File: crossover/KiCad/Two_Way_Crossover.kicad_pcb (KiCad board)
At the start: 2 copper layers, 116.8 x 152.4 mm, 21 parts, among them J1 Conn_01x01_Female, J2 Conn_01x01_Female, J3 Woofer, J4 Tweeter

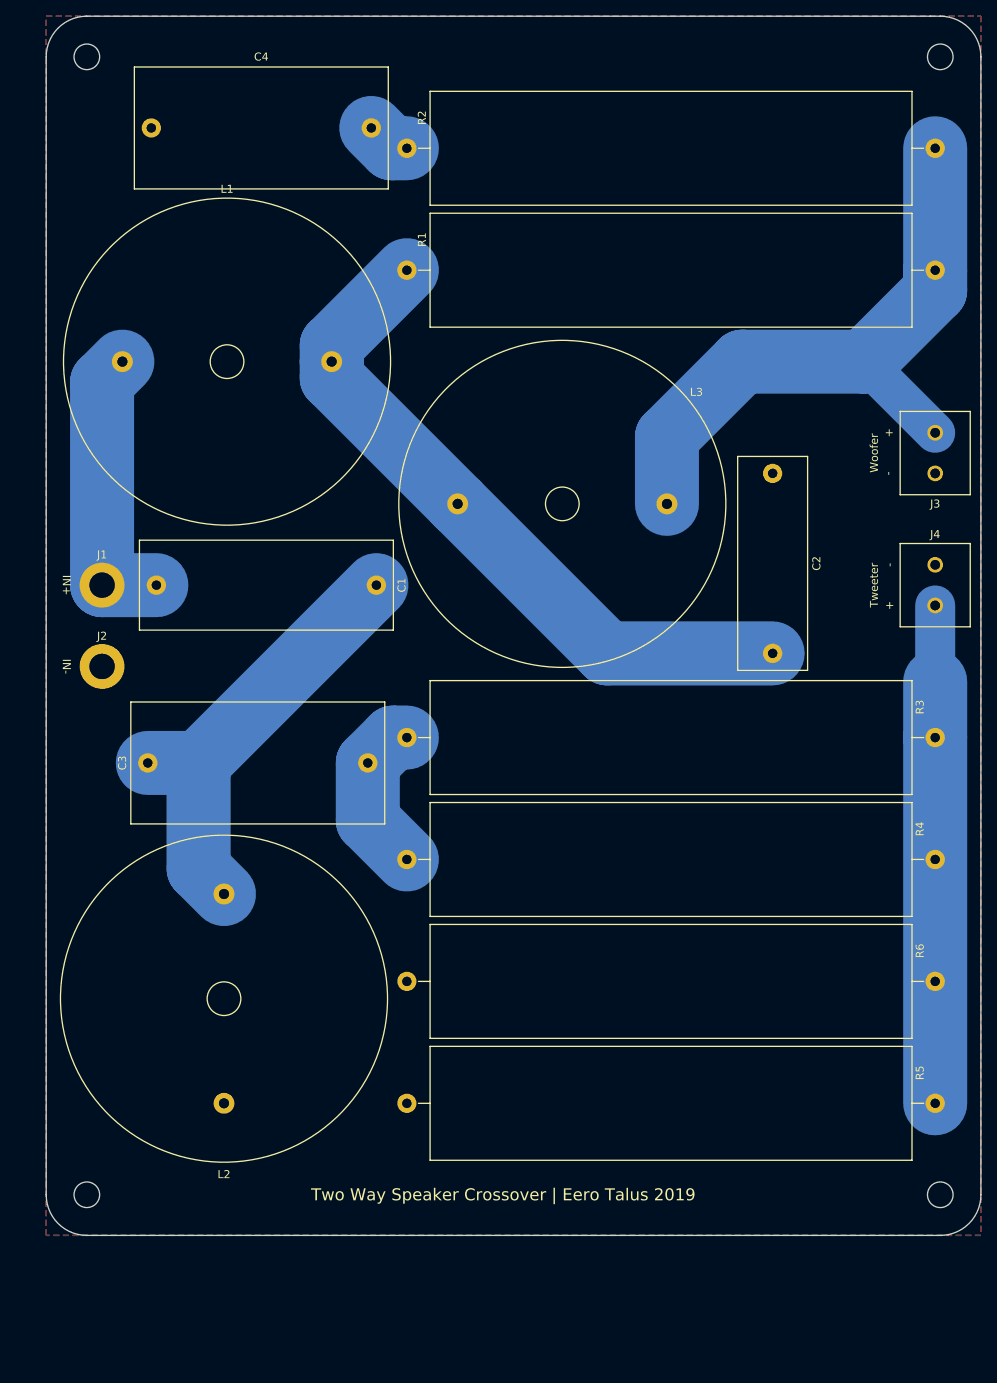
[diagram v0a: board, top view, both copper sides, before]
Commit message: Redesign PCB
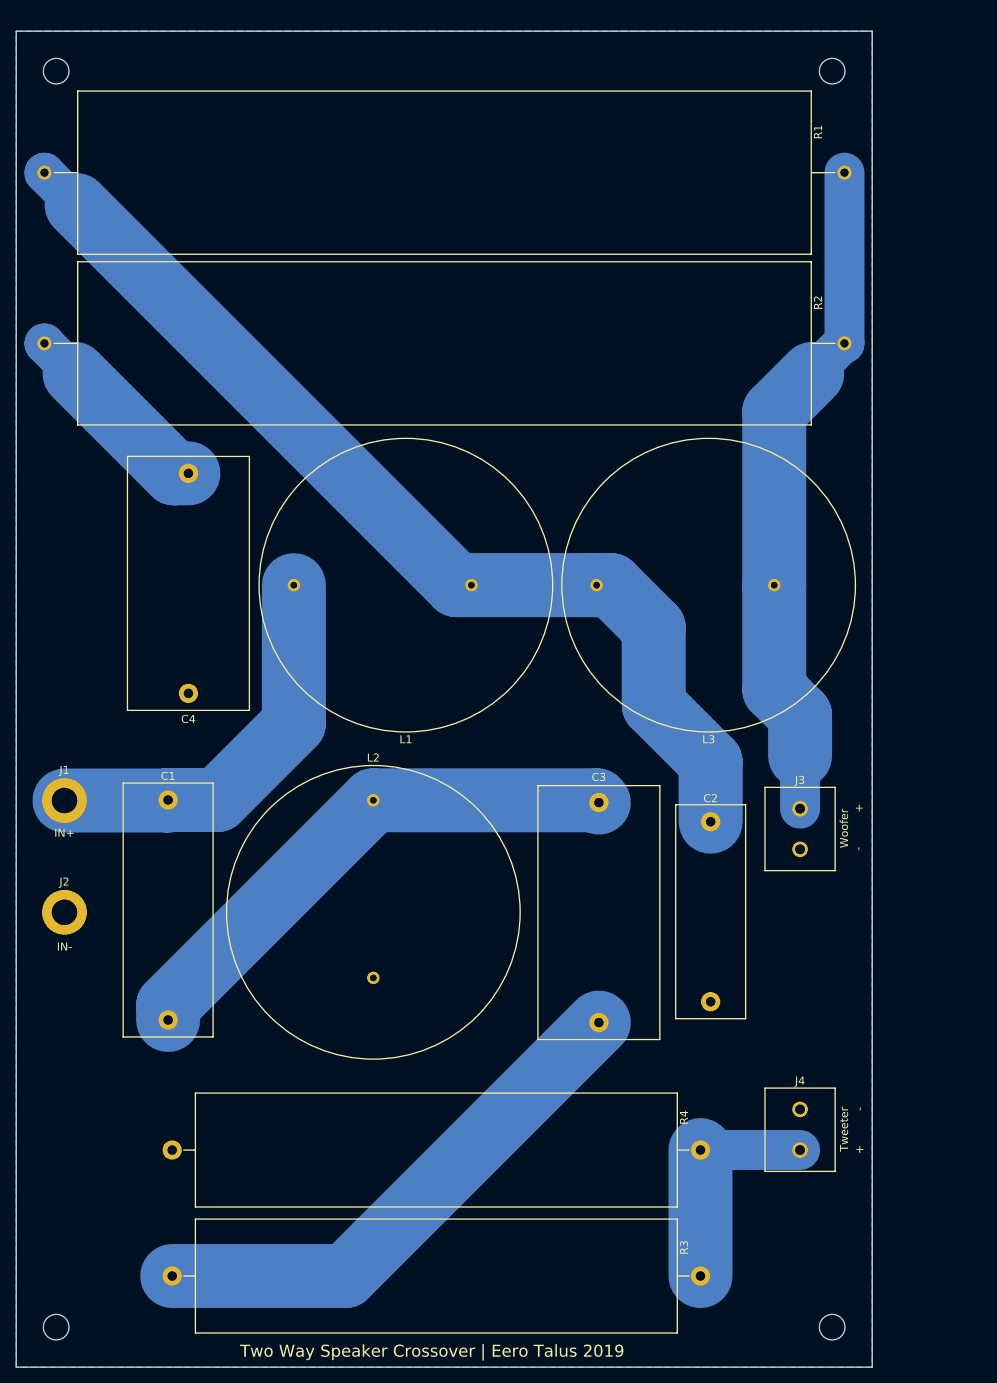
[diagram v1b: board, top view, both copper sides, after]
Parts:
- removed R5, R6: 8R2, Resistor_THT:R_Axial_Power_L60.0mm_W14.0mm_P66.04mm
- L1, L2, L3: footprint Inductor_THT:L_Radial_D40.6mm_P26.16mm_Vishay_IHB-5 -> etal_Inductors:Radial_D36.5mm_H12.0mm_P23.0mm
- R1, R2: footprint Resistor_THT:R_Axial_Power_L60.0mm_W14.0mm_P66.04mm -> etal_Power_Resistor:Resistor_Power_Axial_L91.5_W20.2_H20.2
- R3, R4: value 8R2 -> 4R7
- moved H1 110.5 mm to (33.0, 31.0)
- moved H3 93.2 mm to (130.0, 31.0)
- moved R3 73.4 mm to (113.5, 181.6)
- moved J4 70.1 mm to (126.0, 163.3)
- moved C2 66.5 mm to (114.8, 147.3), turned to 90 degrees
- moved C1 60.3 mm to (47.0, 149.6), turned to 90 degrees
- moved C3 56.6 mm to (100.8, 122.4), turned to 270 degrees
- moved R4 51.6 mm to (113.5, 165.9), turned to 180 degrees
- moved J3 49.9 mm to (126.0, 125.7)
- moved C4 48.9 mm to (49.5, 81.3), turned to 270 degrees
- moved L1 45.1 mm to (76.7, 95.2), turned to 180 degrees
- moved L3 33.0 mm to (114.6, 95.2), turned to 180 degrees
- moved J2 31.1 mm to (34.0, 136.1)
- moved J1 27.3 mm to (34.0, 122.2)
- moved R2 24.8 mm to (81.5, 65.0), turned to 180 degrees
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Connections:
- R4 pad 1: Net-(C3-Pad2) -> Net-(J4-Pad1)
- R4 pad 2: Net-(J4-Pad1) -> GND
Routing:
- net Net-(J4-Pad1): track 108.0 -> 28.2 mm
- net Net-(C3-Pad2): track 20.3 -> 66.5 mm
- net Net-(C2-Pad2): track 86.7 -> 126.9 mm
- net Net-(C4-Pad1): track 5.50 -> 24.8 mm
- net Net-(C1-Pad2): track 35.8 -> 50.0 mm
- net Net-(C1-Pad1): track 55.5 -> 66.4 mm
- net Net-(J3-Pad1): track 79.8 -> 89.7 mm
- removed copper zone on F.Cu, net GND
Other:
- board size 116.8 x 152.4 mm -> 107 x 167 mm
